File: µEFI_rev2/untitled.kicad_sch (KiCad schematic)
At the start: 27 parts, among them U36 MAX9926UAEE+

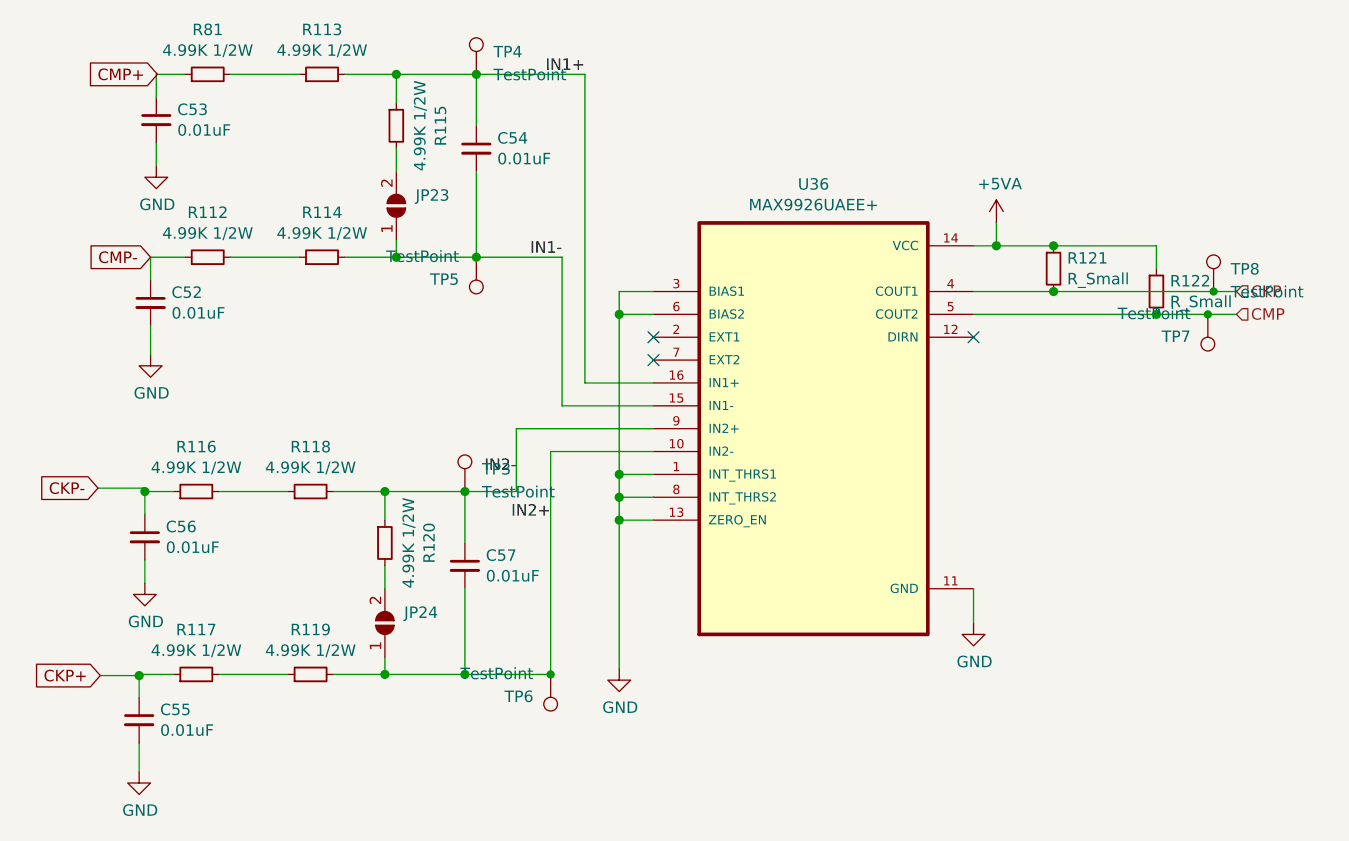
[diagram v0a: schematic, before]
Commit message: bump to kicad 6, init uEFI v3
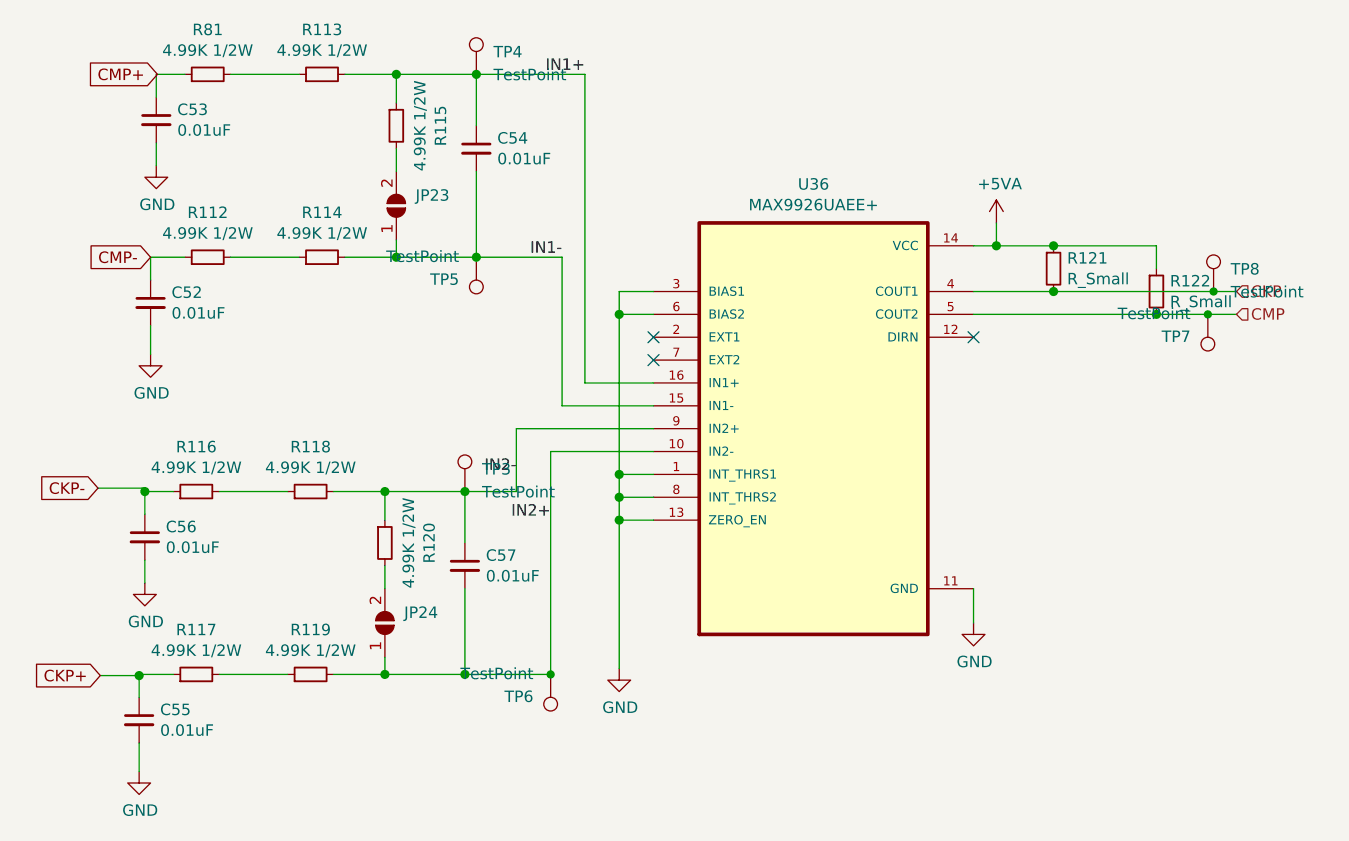
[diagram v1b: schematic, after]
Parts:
- C52, C53, C54, C55, C56, C57: footprint Capacitor_SMD:C_0603_1608Metric -> Capacitor_SMD:C_0805_2012Metric
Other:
- company: (none) -> Churrosoft
- title: (none) -> uEFI

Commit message: move old boards to __old
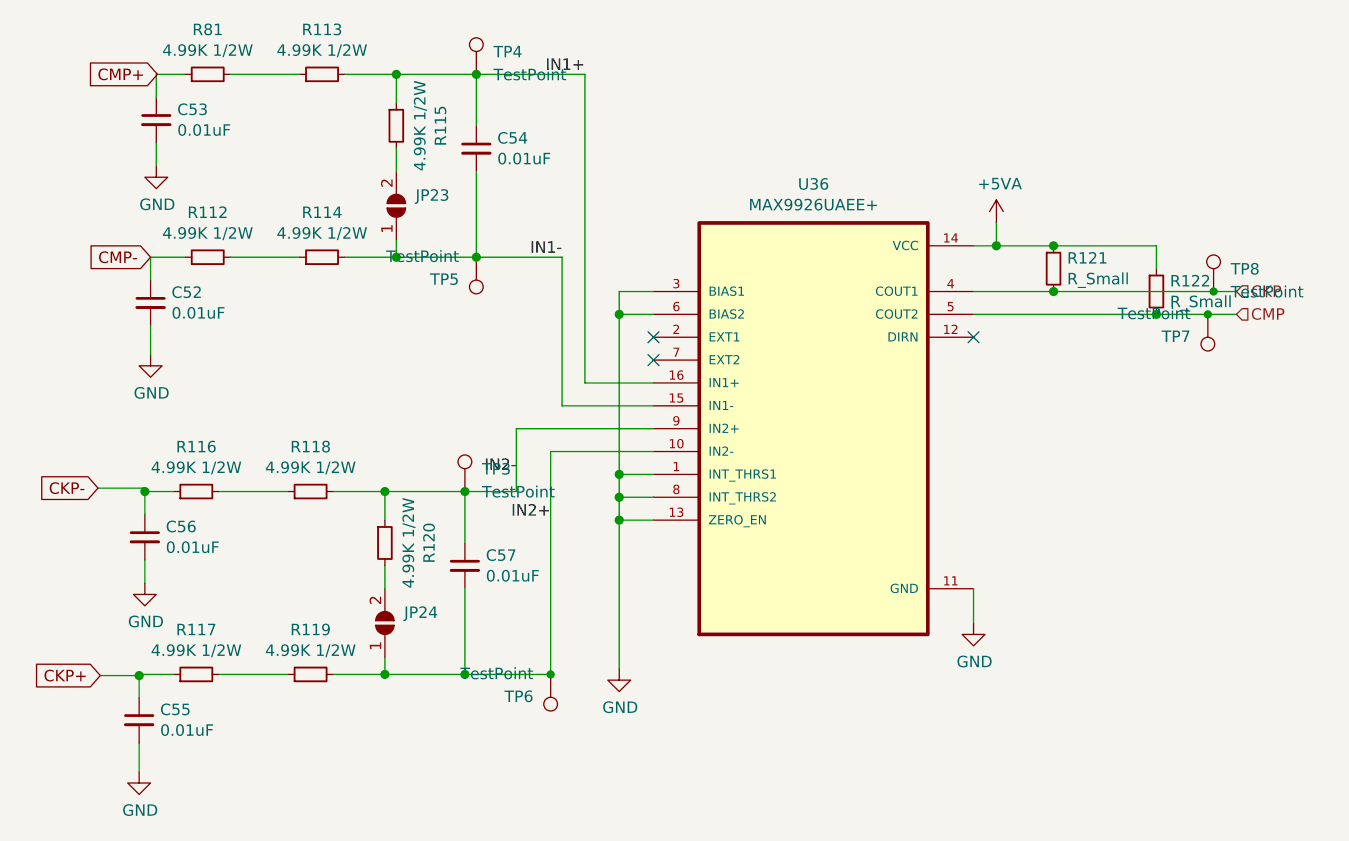
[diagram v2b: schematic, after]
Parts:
- C52, C53, C54, C55, C56, C57: footprint Capacitor_SMD:C_0805_2012Metric -> Capacitor_SMD:C_0603_1608Metric
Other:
- company: Churrosoft -> (none)
- title: uEFI -> (none)
